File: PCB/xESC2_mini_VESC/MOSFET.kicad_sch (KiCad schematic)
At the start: 9 parts, among them J8 Conn_02x02_Counter_Clockwise, Q5 BSC026N08NS5, Q6 BSC026N08NS5

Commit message: BoM data updates
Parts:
- C26: Digikey C-603-1000pF-100V-X7R -> 490-4780-1-ND; Part Number 490-4764-2-ND -> GCM188R72A102KA37D
- J8: LCSC (none) -> C124362; Part Number (none) -> B-2100S04P-B110; Stock_PN (none) -> J-TH-2x2-.1
- R10, R9: Digikey ERJ-3GEYJ2R2V -> P2.2GCT-ND; Part Number P2.2GCT-ND -> ERJ-3GEYJ2R2V
- R11: Digikey (none) -> 738-CSM2512FT33L0CT-ND; Part Number (none) -> ARP2512GJR033
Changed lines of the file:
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@@
+      (effects (font (size 1.27 1.27)) hide)
+    )
+    (property "Part Number" "ARP2512GJR033" (id 6) (at 195.58 83.82 0)
+      (effects (font (size 1.27 1.27)) hide)
+    )
+    (property "Digikey" "738-CSM2512FT33L0CT-ND" (id 7) (at 195.58 83.82 0)
       (effects (font (size 1.27 1.27)) hide)
     )
@@
       (effects (font (size 1.27 1.27)) hide)
     )
-    (property "Digikey" "ERJ-3GEYJ2R2V" (id 4) (at 153.67 71.12 0)
+    (property "Digikey" "P2.2GCT-ND" (id 4) (at 153.67 71.12 0)
       (effects (font (size 1.27 1.27)) hide)
     )
-    (property "Part Number" "P2.2GCT-ND" (id 5) (at 153.67 71.12 0)
+    (property "Part Number" "ERJ-3GEYJ2R2V" (id 5) (at 153.67 71.12 0)
       (effects (font (size 1.27 1.27)) hide)
     )
@@
       (effects (font (size 1.27 1.27)) hide)
     )
-    (property "Digikey" "ERJ-3GEYJ2R2V" (id 4) (at 153.67 96.52 0)
+    (property "Digikey" "P2.2GCT-ND" (id 4) (at 153.67 96.52 0)
       (effects (font (size 1.27 1.27)) hide)
     )
-    (property "Part Number" "P2.2GCT-ND" (id 5) (at 153.67 96.52 0)
+    (property "Part Number" "ERJ-3GEYJ2R2V" (id 5) (at 153.67 96.52 0)
       (effects (font (size 1.27 1.27)) hide)
     )
@@
       (effects (font (size 1.27 1.27)) hide)
     )
-    (property "Digikey" "C-603-1000pF-100V-X7R" (id 4) (at 218.44 101.6 0)
+    (property "Digikey" "490-4780-1-ND" (id 4) (at 218.44 101.6 0)
       (effects (font (size 1.27 1.27)) hide)
     )
-    (property "Part Number" "490-4764-2-ND" (id 5) (at 218.44 101.6 0)
+    (property "Part Number" "GCM188R72A102KA37D" (id 5) (at 218.44 101.6 0)
       (effects (font (size 1.27 1.27)) hide)
     )
@@
       (effects (font (size 1.27 1.27)) hide)
     )
+    (property "LCSC" "C124362" (id 4) (at 236.22 83.82 0)
+      (effects (font (size 1.27 1.27)) hide)
+    )
+    (property "Part Number" "B-2100S04P-B110" (id 5) (at 236.22 83.82 0)
+      (effects (font (size 1.27 1.27)) hide)
+    )
+    (property "Stock_PN" "J-TH-2x2-.1" (id 6) (at 236.22 83.82 0)
+      (effects (font (size 1.27 1.27)) hide)
+    )

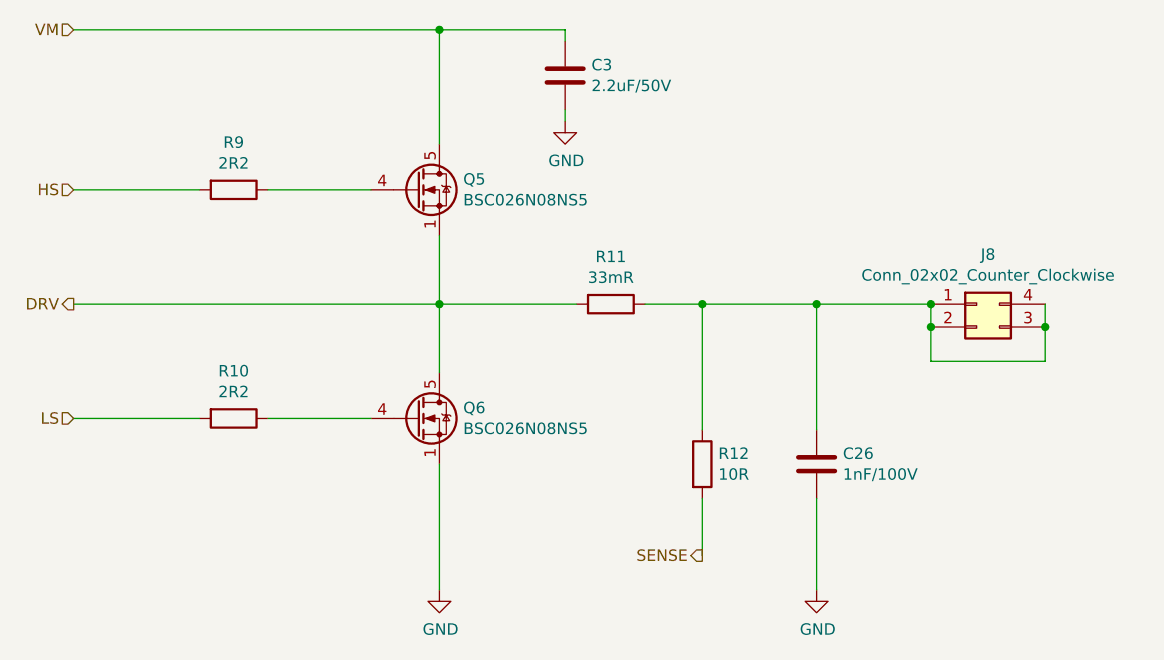
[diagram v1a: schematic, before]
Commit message: updated BOM for .1uF caps
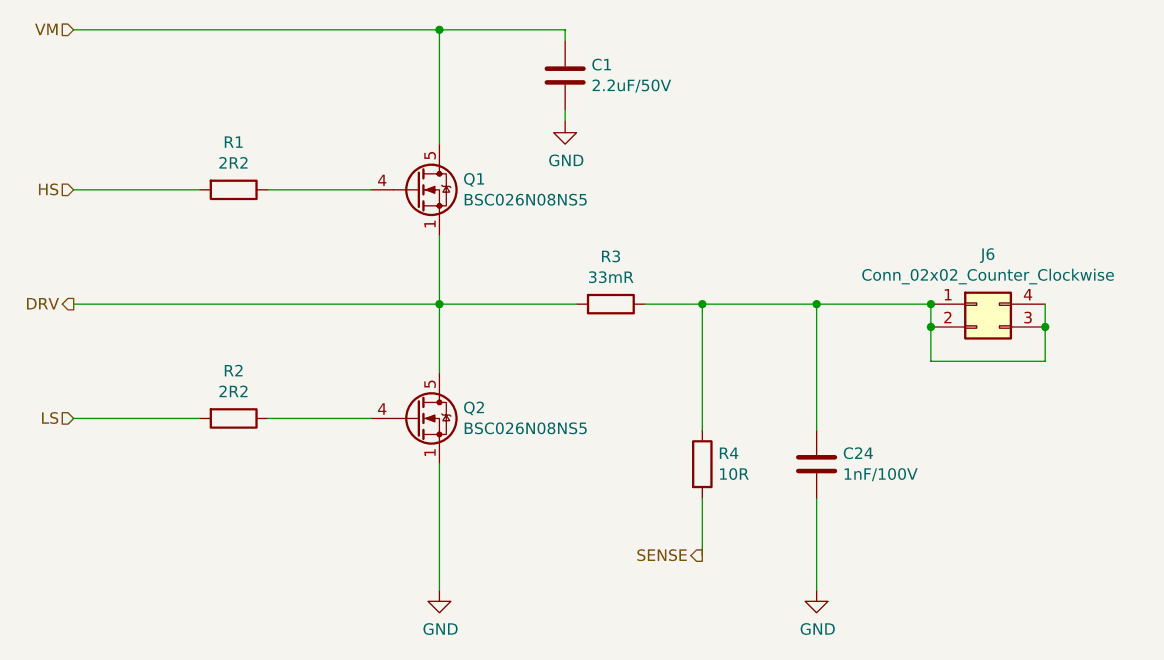
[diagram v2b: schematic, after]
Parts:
- renumbered C3 to C1, C26 to C24, J8 to J6, Q5 to Q1, Q6 to Q2, R9 to R1, R10 to R2, R11 to R3, R12 to R4
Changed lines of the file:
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@@
     (effects (font (size 1.27 1.27)) (justify right))
   )
-  (symbol (lib_id "Transistor_FET:BSC026N08NS5") (at 173.99 71.12 0)
-    (in_bom yes) (on_board yes)
-    (property "Reference" "Q5" (id 0) (at 179.1716 69.9516 0)
+  (symbol (lib_id "Transistor_FET:BSC026N08NS5") (at 173.99 71.12 0) (unit 1)
+    (in_bom yes) (on_board yes)
+    (property "Reference" "Q1" (id 0) (at 179.1716 69.9516 0)
       (effects (font (size 1.27 1.27)) (justify left))
     )
@@
     (pin "5")
   )
-  (symbol (lib_id "Transistor_FET:BSC026N08NS5") (at 173.99 96.52 0)
-    (in_bom yes) (on_board yes)
-    (property "Reference" "Q6" (id 0) (at 179.1716 95.3516 0)
+  (symbol (lib_id "Transistor_FET:BSC026N08NS5") (at 173.99 96.52 0) (unit 1)
+    (in_bom yes) (on_board yes)
+    (property "Reference" "Q2" (id 0) (at 179.1716 95.3516 0)
       (effects (font (size 1.27 1.27)) (justify left))
     )
@@
     (pin "5")
   )
-  (symbol (lib_id "Device:R") (at 195.58 83.82 270)
-    (in_bom yes) (on_board yes)
-    (property "Reference" "R11" (id 0) (at 195.58 78.5622 90))
+  (symbol (lib_id "Device:R") (at 195.58 83.82 270) (unit 1)
+    (in_bom yes) (on_board yes)
+    (property "Reference" "R3" (id 0) (at 195.58 78.5622 90))
     (property "Value" "33mR" (id 1) (at 195.58 80.8736 90))
     (property "Footprint" "Resistor_SMD:R_2512_6332Metric" (id 2) (at 195.58 82.042 90)
@@
     (pin "2")
   )
-  (symbol (lib_id "Device:R") (at 153.67 71.12 270)
-    (in_bom yes) (on_board yes)
-    (property "Reference" "R9" (id 0) (at 153.67 65.8622 90))
+  (symbol (lib_id "Device:R") (at 153.67 71.12 270) (unit 1)
+    (in_bom yes) (on_board yes)
+    (property "Reference" "R1" (id 0) (at 153.67 65.8622 90))
     (property "Value" "2R2" (id 1) (at 153.67 68.1736 90))
     (property "Footprint" "Resistor_SMD:R_0603_1608Metric" (id 2) (at 153.67 69.342 90)
@@
     (pin "2")
   )
-  (symbol (lib_id "Device:R") (at 153.67 96.52 270)
-    (in_bom yes) (on_board yes)
-    (property "Reference" "R10" (id 0) (at 153.67 91.2622 90))
+  (symbol (lib_id "Device:R") (at 153.67 96.52 270) (unit 1)
+    (in_bom yes) (on_board yes)
+    (property "Reference" "R2" (id 0) (at 153.67 91.2622 90))
     (property "Value" "2R2" (id 1) (at 153.67 93.5736 90))
     (property "Footprint" "Resistor_SMD:R_0603_1608Metric" (id 2) (at 153.67 94.742 90)
@@
     (pin "2")
   )
-  (symbol (lib_id "Device:R") (at 205.74 101.6 0)
-    (in_bom yes) (on_board yes)
-    (property "Reference" "R12" (id 0) (at 207.518 100.4316 0)
+  (symbol (lib_id "Device:R") (at 205.74 101.6 0) (unit 1)
+    (in_bom yes) (on_board yes)
+    (property "Reference" "R4" (id 0) (at 207.518 100.4316 0)
       (effects (font (size 1.27 1.27)) (justify left))
     )
@@
     (pin "2")
   )
-  (symbol (lib_id "power:GND") (at 176.53 115.57 0)
-    (in_bom yes) (on_board yes)
-    (property "Reference" "#PWR0105" (id 0) (at 176.53 121.92 0)
+  (symbol (lib_id "power:GND") (at 176.53 115.57 0) (unit 1)
+    (in_bom yes) (on_board yes)
+    (property "Reference" "#PWR0101" (id 0) (at 176.53 121.92 0)
       (effects (font (size 1.27 1.27)) hide)
     )
@@
     (pin "1")
   )
-  (symbol (lib_id "Device:C") (at 190.5 58.42 0)
-    (in_bom yes) (on_board yes)
-    (property "Reference" "C3" (id 0) (at 193.421 57.2516 0)
+  (symbol (lib_id "Device:C") (at 190.5 58.42 0) (unit 1)
+    (in_bom yes) (on_board yes)
+    (property "Reference" "C1" (id 0) (at 193.421 57.2516 0)
       (effects (font (size 1.27 1.27)) (justify left))
     )
@@
     (pin "2")
   )
-  (symbol (lib_id "power:GND") (at 190.5 63.5 0)
-    (in_bom yes) (on_board yes)
-    (property "Reference" "#PWR0106" (id 0) (at 190.5 69.85 0)
+  (symbol (lib_id "power:GND") (at 190.5 63.5 0) (unit 1)
+    (in_bom yes) (on_board yes)
+    (property "Reference" "#PWR0102" (id 0) (at 190.5 69.85 0)
       (effects (font (size 1.27 1.27)) hide)
     )
@@
     (pin "1")
   )
-  (symbol (lib_id "Device:C") (at 218.44 101.6 0)
-    (in_bom yes) (on_board yes)
-    (property "Reference" "C26" (id 0) (at 221.361 100.4316 0)
+  (symbol (lib_id "Device:C") (at 218.44 101.6 0) (unit 1)
+    (in_bom yes) (on_board yes)
+    (property "Reference" "C24" (id 0) (at 221.361 100.4316 0)
       (effects (font (size 1.27 1.27)) (justify left))
     )
@@
     (pin "2")
   )
-  (symbol (lib_id "power:GND") (at 218.44 115.57 0)
-    (in_bom yes) (on_board yes)
-    (property "Reference" "#PWR0118" (id 0) (at 218.44 121.92 0)
+  (symbol (lib_id "power:GND") (at 218.44 115.57 0) (unit 1)
+    (in_bom yes) (on_board yes)
+    (property "Reference" "#PWR0116" (id 0) (at 218.44 121.92 0)
       (effects (font (size 1.27 1.27)) hide)
     )
@@
     (pin "1")
   )
-  (symbol (lib_id "Connector_Generic:Conn_02x02_Counter_Clockwise") (at 236.22 83.82 0)
-    (in_bom yes) (on_board yes)
-    (property "Reference" "J8" (id 0) (at 237.49 78.3082 0))
+  (symbol (lib_id "Connector_Generic:Conn_02x02_Counter_Clockwise") (at 236.22 83.82 0) (unit 1)
+    (in_bom yes) (on_board yes)
+    (property "Reference" "J6" (id 0) (at 237.49 78.3082 0))
     (property "Value" "Conn_02x02_Counter_Clockwise" (id 1) (at 237.49 80.6196 0))
     (property "Footprint" "Connector_PinHeader_2.54mm:PinHeader_2x02_P2.54mm_Vertical" (id 2) (at 236.22 83.82 0)

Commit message: updated wrong BOM part number
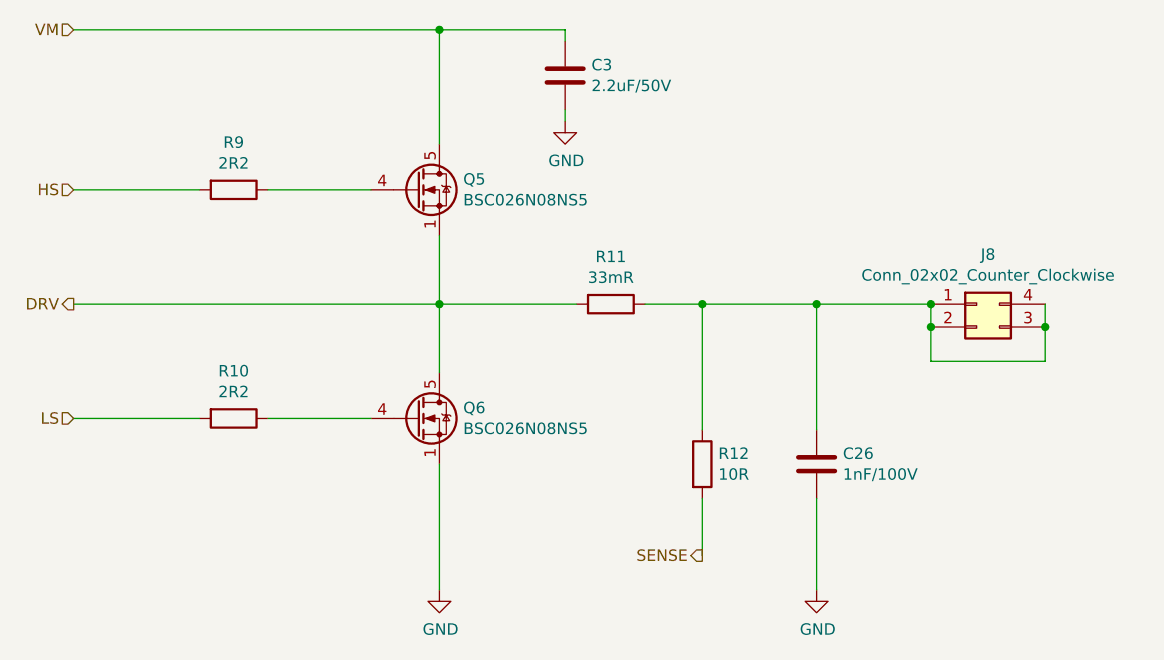
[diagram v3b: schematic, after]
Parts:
- renumbered C24 to C26, C1 to C3, J6 to J8, Q1 to Q5, Q2 to Q6, R2 to R10, R3 to R11, R4 to R12, R1 to R9
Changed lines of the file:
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@@
     (effects (font (size 1.27 1.27)) (justify right))
   )
-  (symbol (lib_id "Transistor_FET:BSC026N08NS5") (at 173.99 71.12 0) (unit 1)
-    (in_bom yes) (on_board yes)
-    (property "Reference" "Q1" (id 0) (at 179.1716 69.9516 0)
+  (symbol (lib_id "Transistor_FET:BSC026N08NS5") (at 173.99 71.12 0)
+    (in_bom yes) (on_board yes)
+    (property "Reference" "Q5" (id 0) (at 179.1716 69.9516 0)
       (effects (font (size 1.27 1.27)) (justify left))
     )
@@
     (pin "5")
   )
-  (symbol (lib_id "Transistor_FET:BSC026N08NS5") (at 173.99 96.52 0) (unit 1)
-    (in_bom yes) (on_board yes)
-    (property "Reference" "Q2" (id 0) (at 179.1716 95.3516 0)
+  (symbol (lib_id "Transistor_FET:BSC026N08NS5") (at 173.99 96.52 0)
+    (in_bom yes) (on_board yes)
+    (property "Reference" "Q6" (id 0) (at 179.1716 95.3516 0)
       (effects (font (size 1.27 1.27)) (justify left))
     )
@@
     (pin "5")
   )
-  (symbol (lib_id "Device:R") (at 195.58 83.82 270) (unit 1)
-    (in_bom yes) (on_board yes)
-    (property "Reference" "R3" (id 0) (at 195.58 78.5622 90))
+  (symbol (lib_id "Device:R") (at 195.58 83.82 270)
+    (in_bom yes) (on_board yes)
+    (property "Reference" "R11" (id 0) (at 195.58 78.5622 90))
     (property "Value" "33mR" (id 1) (at 195.58 80.8736 90))
     (property "Footprint" "Resistor_SMD:R_2512_6332Metric" (id 2) (at 195.58 82.042 90)
@@
     (pin "2")
   )
-  (symbol (lib_id "Device:R") (at 153.67 71.12 270) (unit 1)
-    (in_bom yes) (on_board yes)
-    (property "Reference" "R1" (id 0) (at 153.67 65.8622 90))
+  (symbol (lib_id "Device:R") (at 153.67 71.12 270)
+    (in_bom yes) (on_board yes)
+    (property "Reference" "R9" (id 0) (at 153.67 65.8622 90))
     (property "Value" "2R2" (id 1) (at 153.67 68.1736 90))
     (property "Footprint" "Resistor_SMD:R_0603_1608Metric" (id 2) (at 153.67 69.342 90)
@@
     (pin "2")
   )
-  (symbol (lib_id "Device:R") (at 153.67 96.52 270) (unit 1)
-    (in_bom yes) (on_board yes)
-    (property "Reference" "R2" (id 0) (at 153.67 91.2622 90))
+  (symbol (lib_id "Device:R") (at 153.67 96.52 270)
+    (in_bom yes) (on_board yes)
+    (property "Reference" "R10" (id 0) (at 153.67 91.2622 90))
     (property "Value" "2R2" (id 1) (at 153.67 93.5736 90))
     (property "Footprint" "Resistor_SMD:R_0603_1608Metric" (id 2) (at 153.67 94.742 90)
@@
     (pin "2")
   )
-  (symbol (lib_id "Device:R") (at 205.74 101.6 0) (unit 1)
-    (in_bom yes) (on_board yes)
-    (property "Reference" "R4" (id 0) (at 207.518 100.4316 0)
+  (symbol (lib_id "Device:R") (at 205.74 101.6 0)
+    (in_bom yes) (on_board yes)
+    (property "Reference" "R12" (id 0) (at 207.518 100.4316 0)
       (effects (font (size 1.27 1.27)) (justify left))
     )
@@
     (pin "2")
   )
-  (symbol (lib_id "power:GND") (at 176.53 115.57 0) (unit 1)
-    (in_bom yes) (on_board yes)
-    (property "Reference" "#PWR0101" (id 0) (at 176.53 121.92 0)
+  (symbol (lib_id "power:GND") (at 176.53 115.57 0)
+    (in_bom yes) (on_board yes)
+    (property "Reference" "#PWR0105" (id 0) (at 176.53 121.92 0)
       (effects (font (size 1.27 1.27)) hide)
     )
@@
     (pin "1")
   )
-  (symbol (lib_id "Device:C") (at 190.5 58.42 0) (unit 1)
-    (in_bom yes) (on_board yes)
-    (property "Reference" "C1" (id 0) (at 193.421 57.2516 0)
+  (symbol (lib_id "Device:C") (at 190.5 58.42 0)
+    (in_bom yes) (on_board yes)
+    (property "Reference" "C3" (id 0) (at 193.421 57.2516 0)
       (effects (font (size 1.27 1.27)) (justify left))
     )
@@
     (pin "2")
   )
-  (symbol (lib_id "power:GND") (at 190.5 63.5 0) (unit 1)
-    (in_bom yes) (on_board yes)
-    (property "Reference" "#PWR0102" (id 0) (at 190.5 69.85 0)
+  (symbol (lib_id "power:GND") (at 190.5 63.5 0)
+    (in_bom yes) (on_board yes)
+    (property "Reference" "#PWR0106" (id 0) (at 190.5 69.85 0)
       (effects (font (size 1.27 1.27)) hide)
     )
@@
     (pin "1")
   )
-  (symbol (lib_id "Device:C") (at 218.44 101.6 0) (unit 1)
-    (in_bom yes) (on_board yes)
-    (property "Reference" "C24" (id 0) (at 221.361 100.4316 0)
+  (symbol (lib_id "Device:C") (at 218.44 101.6 0)
+    (in_bom yes) (on_board yes)
+    (property "Reference" "C26" (id 0) (at 221.361 100.4316 0)
       (effects (font (size 1.27 1.27)) (justify left))
     )
@@
     (pin "2")
   )
-  (symbol (lib_id "power:GND") (at 218.44 115.57 0) (unit 1)
-    (in_bom yes) (on_board yes)
-    (property "Reference" "#PWR0116" (id 0) (at 218.44 121.92 0)
+  (symbol (lib_id "power:GND") (at 218.44 115.57 0)
+    (in_bom yes) (on_board yes)
+    (property "Reference" "#PWR0118" (id 0) (at 218.44 121.92 0)
       (effects (font (size 1.27 1.27)) hide)
     )
@@
     (pin "1")
   )
-  (symbol (lib_id "Connector_Generic:Conn_02x02_Counter_Clockwise") (at 236.22 83.82 0) (unit 1)
-    (in_bom yes) (on_board yes)
-    (property "Reference" "J6" (id 0) (at 237.49 78.3082 0))
+  (symbol (lib_id "Connector_Generic:Conn_02x02_Counter_Clockwise") (at 236.22 83.82 0)
+    (in_bom yes) (on_board yes)
+    (property "Reference" "J8" (id 0) (at 237.49 78.3082 0))
     (property "Value" "Conn_02x02_Counter_Clockwise" (id 1) (at 237.49 80.6196 0))
     (property "Footprint" "Connector_PinHeader_2.54mm:PinHeader_2x02_P2.54mm_Vertical" (id 2) (at 236.22 83.82 0)
